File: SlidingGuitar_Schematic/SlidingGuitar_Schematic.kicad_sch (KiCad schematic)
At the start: 13 parts, among them J1 Barrel_Jack, M1 Motor_DC, U1 DRV8871DDA, U2 LM386, U3 VTL5C

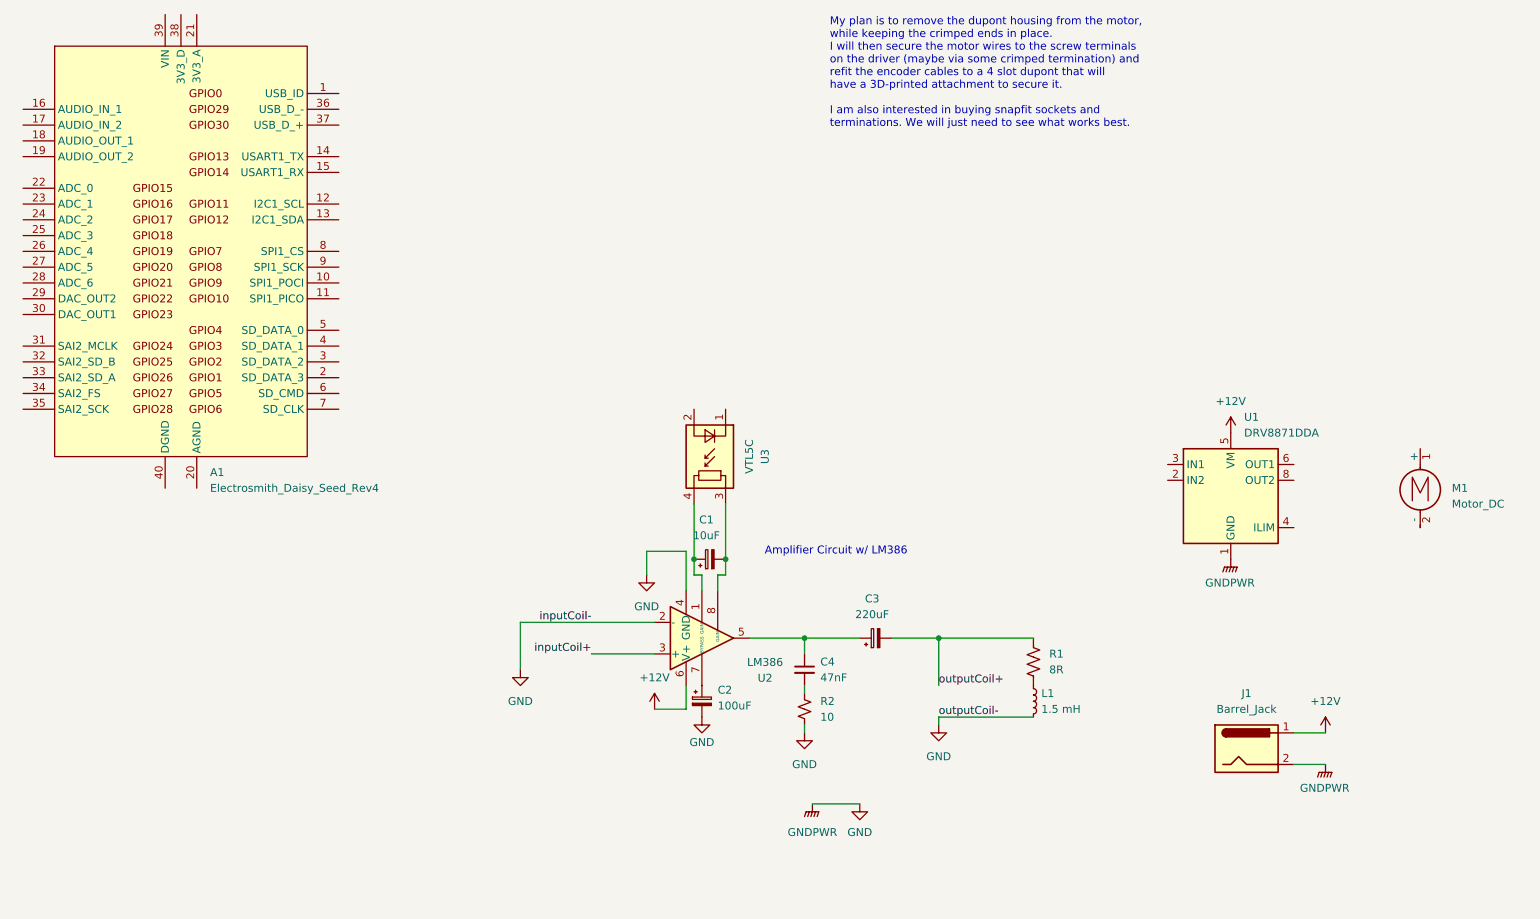
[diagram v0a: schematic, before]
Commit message: Add lock file for SlidingGuitar_Schematic to track PCB design session
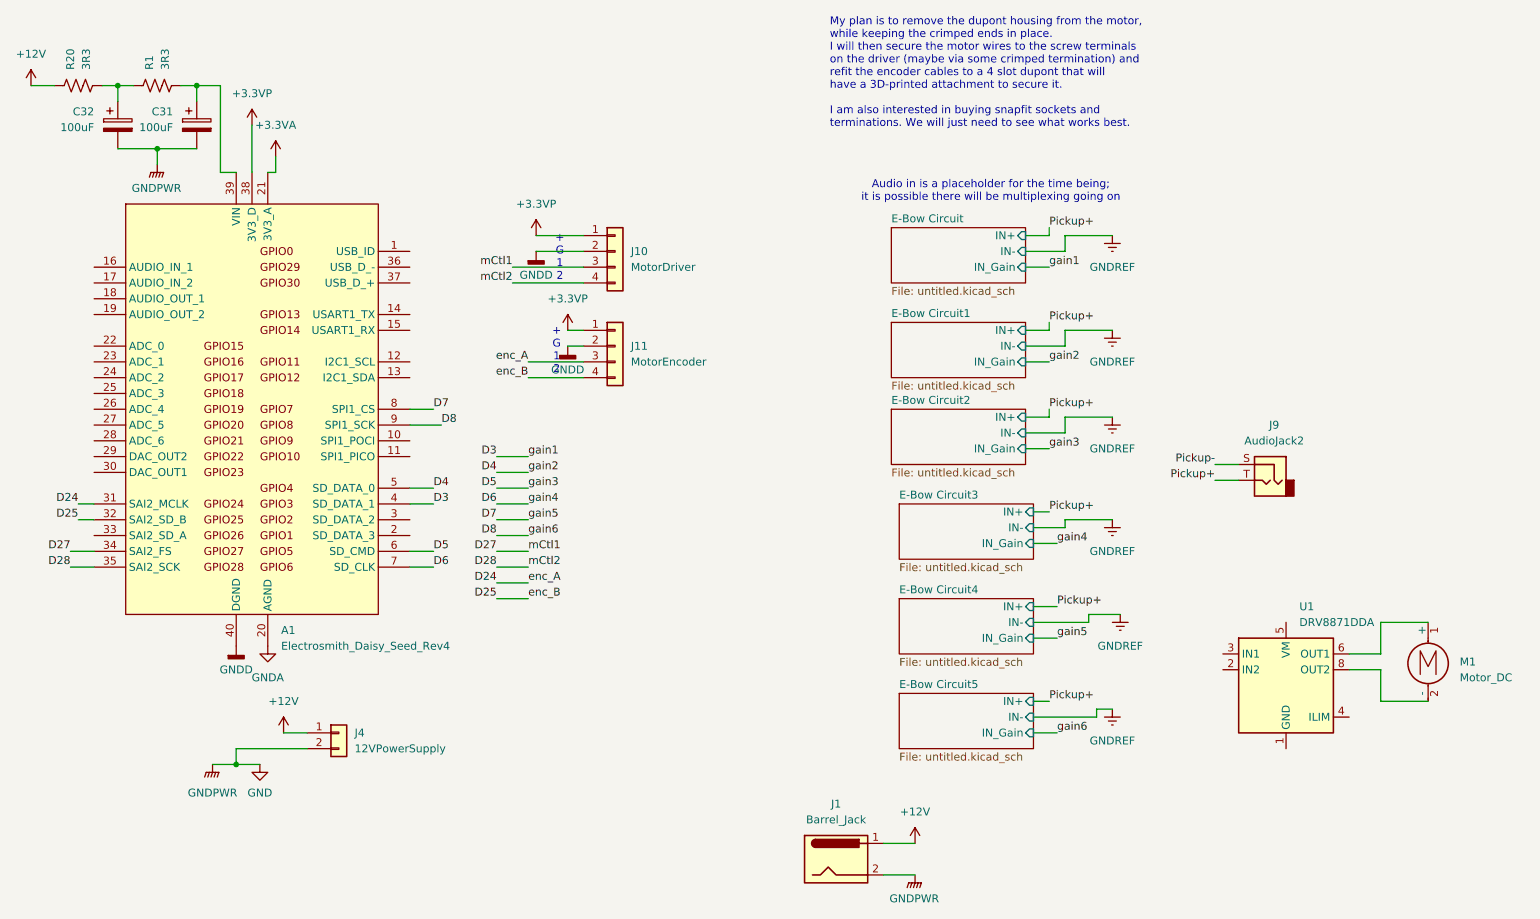
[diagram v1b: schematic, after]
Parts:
- removed C1: 10uF, symbol Device:C_Polarized_Small
- removed C2: 100uF, symbol Device:C_Polarized_Small
- removed C3: 220uF, symbol Device:C_Polarized_Small
- removed C4: 47nF, symbol Device:C_Small
- removed L1: 1.5 mH, symbol Device:L_Small
- removed R2: 10, symbol Device:R_Small_US
- removed U2: LM386, Package_DIP:DIP-8_W7.62mm, symbol Amplifier_Audio:LM386
- removed U3: VTL5C, OptoDevice:PerkinElmer_VTL5Cx2, symbol Isolator:VTL5C
- added C31, C32: 100uF, Capacitor_THT:CP_Radial_D8.0mm_P5.00mm, symbol Device:C_Polarized
- added J10: MotorDriver, Connector_PinHeader_2.54mm:PinHeader_1x04_P2.54mm_Vertical, symbol Connector_Generic:Conn_01x04
- added J11: MotorEncoder, Connector_PinHeader_2.54mm:PinHeader_1x04_P2.54mm_Vertical, symbol Connector_Generic:Conn_01x04
- added J4: 12VPowerSupply, Connector_PinHeader_2.54mm:PinHeader_1x02_P2.54mm_Vertical, symbol Connector_Generic:Conn_01x02
- added J9: AudioJack2, symbol Connector_Audio:AudioJack2
- added R20: 3R3, Resistor_THT:R_Axial_DIN0207_L6.3mm_D2.5mm_P7.62mm_Horizontal, symbol Device:R_US
- J1: footprint (none) -> Connector_BarrelJack:BarrelJack_Horizontal
- R1: value 8R -> 3R3; footprint (none) -> Resistor_THT:R_Axial_DIN0207_L6.3mm_D2.5mm_P7.62mm_Horizontal
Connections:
- net +12V: now also J4.1 (Pin_1), R20.1; no longer U1.5 (VM)
- net GND: now also C31.2, C32.2, J4.2 (Pin_2); no longer U1.1 (GND), U1.7 (GND), U1.9 (GND)
- net at M1.1 (+): now also U1.6 (OUT1)
- net at M1.2 (-): now also U1.8 (OUT2)
- net GNDA: now reaches A1.20 (AGND)
- net +3.3VA: now reaches A1.21 (3V3_A)
- net D24: now reaches A1.31 (SAI2_MCLK)
- net D24: now also J11.3 (Pin_3)
- net D25: now reaches A1.32 (SAI2_SD_B)
- net D25: now also J11.4 (Pin_4)
- net D27: now reaches A1.34 (SAI2_FS)
- net D27: now also J10.3 (Pin_3)
- net D28: now reaches A1.35 (SAI2_SCK)
- net D28: now also J10.4 (Pin_4)
- net +3.3VP: now reaches A1.38 (3V3_D)
- net +3.3VP: now also J10.1 (Pin_1), J11.1 (Pin_1)
- net at A1.39 (VIN): now also R1.2, C31.1
- net D3: now reaches A1.4 (SD_DATA_1)
- net GNDD: now reaches A1.40 (DGND)
- net GNDD: now also J10.2 (Pin_2), J11.2 (Pin_2)
- net D4: now reaches A1.5 (SD_DATA_0)
- net D5: now reaches A1.6 (SD_CMD)
- net D6: now reaches A1.7 (SD_CLK)
- net D7: now reaches A1.8 (SPI1_CS)
- net D8: now reaches A1.9 (SPI1_SCK)
- net outputCoil+: no longer names the net of R1.1
- net outputCoil+: now also C32.1, R20.2
- new net: U1.1 (GND), U1.7 (GND), U1.9 (GND)
- new net Pickup+: J9.T
- new net Pickup-: J9.S
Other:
- added sheet E-Bow Circuit (untitled.kicad_sch)
- added sheet E-Bow Circuit1 (untitled.kicad_sch)
- added sheet E-Bow Circuit2 (untitled.kicad_sch)
- added sheet E-Bow Circuit3 (untitled.kicad_sch)
- added sheet E-Bow Circuit4 (untitled.kicad_sch)
- added sheet E-Bow Circuit5 (untitled.kicad_sch)
- note added: "+ G 1 2"
- note added: "Audio in is a placeholder for the time being; it is possible there will be multiplexing going on"
- note removed: "Amplifier Circuit w/ LM386"
- moved on the sheet: A1, J1, M1, U1
